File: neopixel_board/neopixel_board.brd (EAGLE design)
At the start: 94 x 86 mm, 64 parts, among them U1 UA7805CKCT, U2 MIC5219, U3 ATMEGA32U4, U4 UA7805CKCT, U5 UA7805CKCT, U6 UA7805CKCT, Y1 16MHz

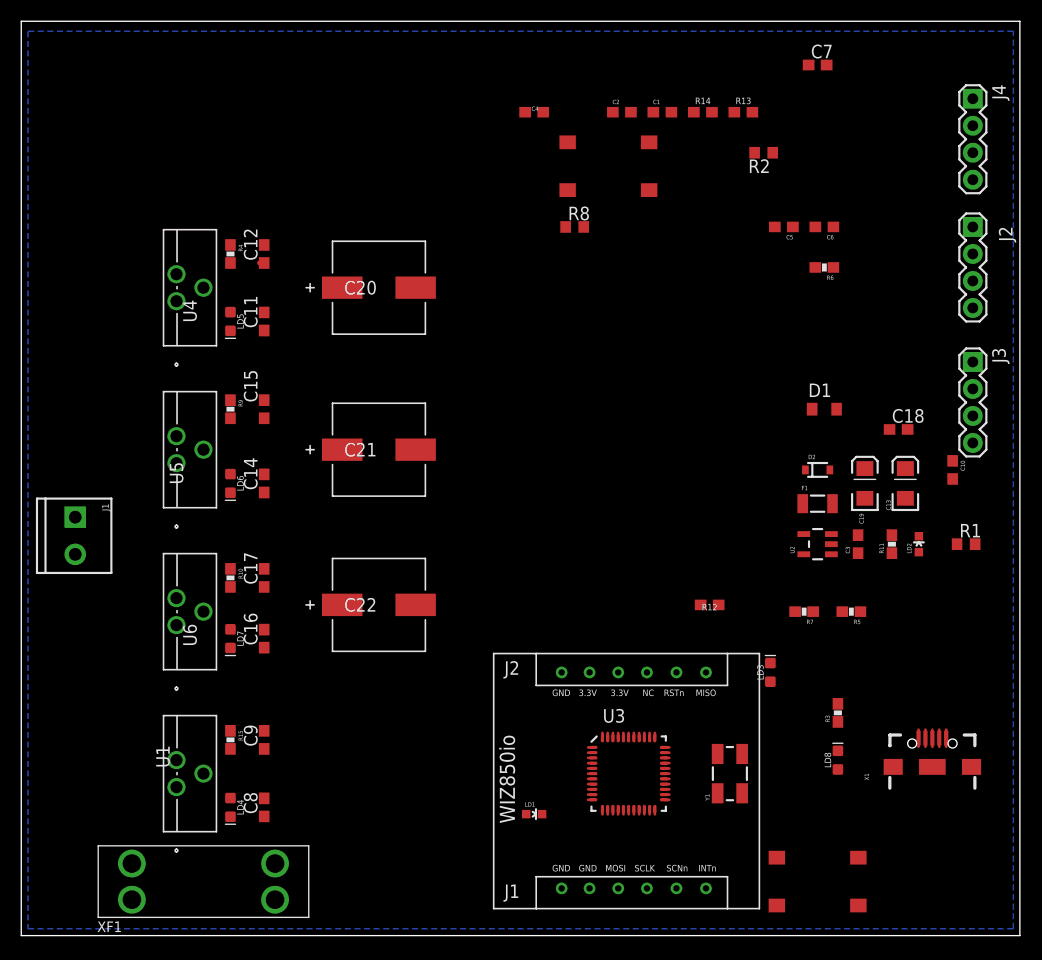
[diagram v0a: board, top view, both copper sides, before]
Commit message: Board Finished (tentative)
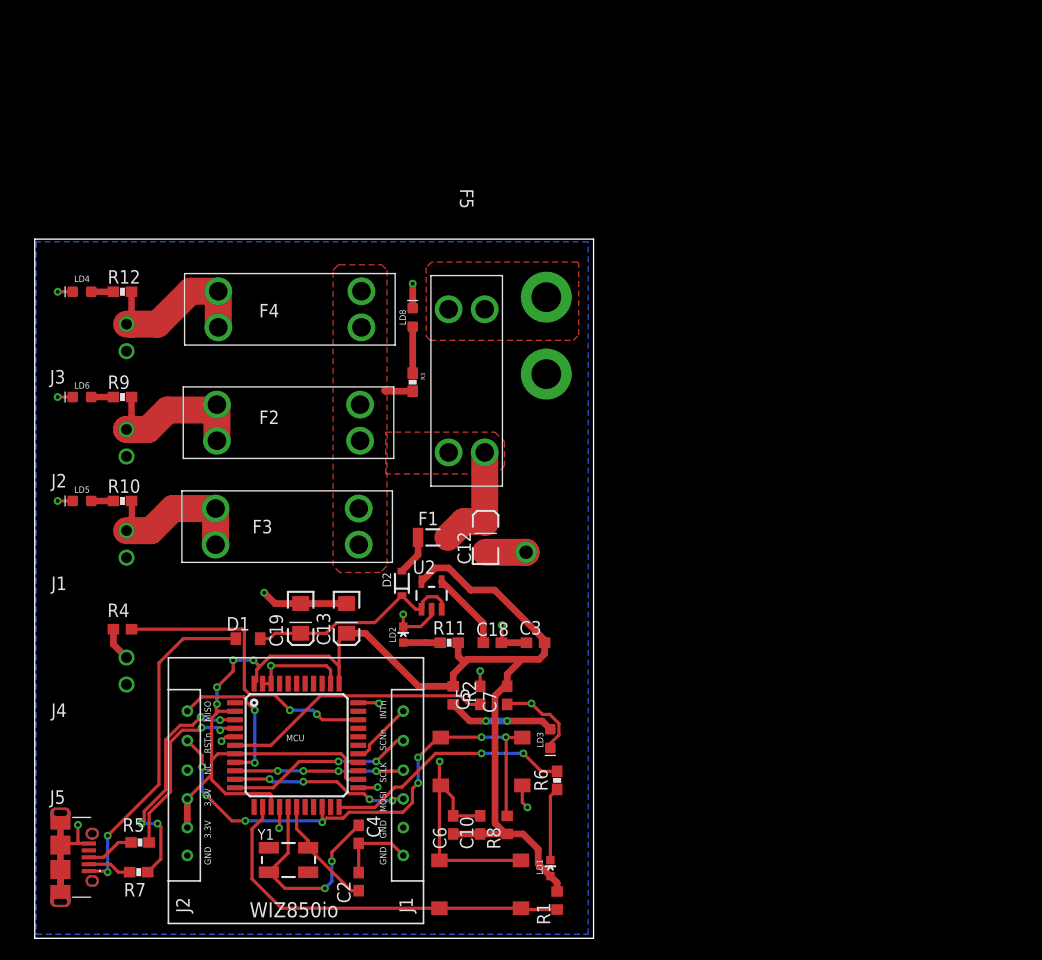
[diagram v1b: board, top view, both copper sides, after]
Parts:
- removed C1: 0.1uF, rcl:C0603
- removed C11, C14, C16, C8: 0.1 uF, rcl:C0603
- removed C15, C17, C9: 0.33 uF, rcl:C0603
- removed C20, C21, C22: 1000uF, neopixel_board:PCAP_8X10-ELECT
- removed LD7: GREEN, SparkFun-LED:LED-0603
- removed R13, R14: 470Ω, SparkFun-Resistors:0603
- removed R15: 1kΩ, SparkFun:0603-RES
- removed U1, U4, U5, U6: UA7805CKCT, Training_Board:KC3
- removed U3: ATMEGA32U4, Testing:QFN-44-NOPAD_1:1-OUTFAKES
- removed X1: (no value), Testing:USB-AB-MICRO-SMD-V03-IN&OUT
- removed XF1: 4A, RoboJackets-Fuses:3557-2
- added 5VSOURCE, GND_TERMINAL: THOLE_SOURCE, neopixel_board:THOLE_SOURCE
- added F2, F3, F4: 4A, neopixel_board:3557-2
- added F5: 13A, neopixel_board:3557-2
- added J5: 47589-0001_2, neopixel_board:MOLEX_47589-0001_FIX
- added MCU: 32U4, SparkFun-IC-Microcontroller:TQFP44
- C12: value 0.33 uF -> 1000uF; device rcl:C0603 -> SparkFun:EIA3216
- J1: value (none) -> SSW-102-02-T-S-RA; device SparkFun-Connectors:SCREWTERMINAL-3.5MM-2 -> neopixel_board:CON2_1X2_TR_SSQ
- J2, J3, J4: value (none) -> SSW-102-02-T-S-RA; device SparkFun-Connectors:1X04 -> neopixel_board:CON2_1X2_TR_SSQ
- R12: value 470Ω -> 1kΩ; device SparkFun-Resistors:0603 -> SparkFun:0603-RES
- R4: value 1kΩ -> 470Ω; device SparkFun:0603-RES -> SparkFun-Resistors:0603
- moved J4 96.1 mm to (9.91, 24.9), turned to 90 degrees
- moved J2 82.2 mm to (9.91, 46.4), turned to 90 degrees
- moved J3 79.7 mm to (9.91, 56.3), turned to 90 degrees
- moved C2 76.5 mm to (31.8, 5.08), turned to 90 degrees
- moved R5 70.4 mm to (11.2, 8.76)
- moved C4 69.9 mm to (31.8, 9.53), turned to 270 degrees
- moved R7 67.2 mm to (11.0, 5.97)
- moved C6 66.2 mm to (40.6, 10.4), turned to 90 degrees
- moved C7 66.1 mm to (45.7, 22.6), turned to 270 degrees
- moved R12 62.6 mm to (9.53, 60.6)
- moved R2 58.8 mm to (40.6, 22.6), turned to 270 degrees
- moved D1 58.4 mm to (21.3, 27.9), turned to 180 degrees
- moved LD8 57.8 mm to (36.8, 58.2)
- moved PB2 57.3 mm to (43.3, 16.4)
- moved R8 56.6 mm to (45.7, 10.4), turned to 90 degrees
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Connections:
- removed net AREF: C1.1, U3.42
- removed net N$3: J4.3, R14.1
- removed net NEOPIXEL_1: R13.2, U3.29
- removed net NEOPIXEL_2: R14.2, U3.30
- removed net UVCC: D1.A, X1.VBUS1
- removed net VCC1: C6.1, C9.1, F1.1, R15.1, U1.3, U3.2, U3.7
- removed net VCC2: C12.1, C20.1, J2.4, R4.1, U4.3
- removed net VCC3: C15.1, C21.1, J3.4, R9.1, U5.3
- removed net VCC4: C17.1, C22.1, J4.4, R10.1, U6.3
- removed net VSOURCE: C11.1, C14.1, C16.1, C8.1, R3.2, U1.1, U4.1, U5.1, U6.1, XF1.3, XF1.4
- new net 5VIN: 5VSOURCE.1, F5.1, F5.2
- new net N$17: D1.A, J5.1
- new net N$18: LD3.A, R2.2
- new net VCC_5V: C12.A, F1.1, F2.3, F2.4, F3.3, F3.4, F4.3, F4.4, F5.3, F5.4, R3.2
- net D+: now also MCU.4; no longer U3.4
- net D-: now also MCU.3; no longer U3.3
- net ETH_INT: now also MCU.27; no longer U3.27
- net ETH_MISO: now also MCU.8; no longer U3.8
- net ETH_MOSI: now also MCU.10; no longer U3.10
- net ETH_RST: now also MCU.20; no longer U3.20
- net ETH_SCK: now also MCU.9; no longer U3.9
- net ETH_SCNN: now also MCU.11; no longer U3.11
- net GND: now also C12.C, GND_TERMINAL.1, J5.5, J5.P$3, J5.P$4, J5.P$5, J5.P$6, MCU.15, MCU.23, MCU.33, MCU.35, MCU.42, MCU.43, MCU.5; no longer C1.2, C11.2, C12.2, C14.2, C15.2, C16.2, C17.2, C20.2, C21.2, C22.2, C8.2, C9.2, J2.2, J3.2, J4.2, LD3.A, LD7.C, R2.2, U1.2, U3.15, U3.23, U3.33, U3.35, U3.43, U3.5, U4.2, U5.2, U6.2, X1.GND1
- net MCU_RST: now also MCU.13; no longer U3.13
- net N$1: now also MCU.16; no longer U3.16
- net N$10: now also F2.1, F2.2, J2.2, R9.2; no longer LD7.A, R10.2
- net N$11: now also F3.1, F3.2, J1.2, R10.2; no longer LD4.A, R15.2
- net N$12: now also F4.1, F4.2, J3.2, R12.2; no longer LD5.A, R4.2
- net N$13: now also J4.2, R4.1; no longer LD6.A, R9.2
- net N$14: now also LD4.A; no longer J2.3
- net N$15: now also LD5.A, R10.1; no longer J3.3, R13.1
- net N$16: now also LD6.A, R9.1; no longer J1.2, XF1.1, XF1.2
- net N$2: now also MCU.17; no longer U3.17
- net N$4: now also MCU.6; no longer U3.6
- net N$6: now also J5.2; no longer X1.D-1
- net N$8: now also J5.3; no longer X1.D+1
- net NEOPIXEL_0: now also MCU.31, R4.2; no longer R12.2, U3.31
- net TXLED: now also MCU.22; no longer U3.22
- net VCC1_3.3V: now also C6.1, MCU.14, MCU.2, MCU.24, MCU.34, MCU.44, MCU.7; no longer U3.14, U3.24, U3.34, U3.44
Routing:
- net VCC1_3.3V: track 0.00 -> 134.1 mm, vias 0 -> 4
- net GND: track 0.00 -> 100.9 mm, vias 0 -> 18
- net ETH_RST: track 0.00 -> 51.0 mm, vias 0 -> 8
- net MCU_RST: track 0.00 -> 37.1 mm
- net N$17: track 0.00 -> 31.7 mm, vias 0 -> 2
- net NEOPIXEL_0: track 0.00 -> 28.1 mm, vias 0 -> 2
- net N$4: track 0.00 -> 25.3 mm
- net TXLED: track 0.00 -> 23.3 mm, vias 0 -> 2
- net D-: track 0.00 -> 23.1 mm, vias 0 -> 4
- net RAW: track 0.00 -> 21.0 mm
- net N$1: track 0.00 -> 20.0 mm, vias 0 -> 2
- net ETH_SCNN: track 0.00 -> 17.7 mm, vias 0 -> 2
- net D+: track 0.00 -> 17.2 mm, vias 0 -> 2
- net ETH_MOSI: track 0.00 -> 16.8 mm, vias 0 -> 4
- net N$10: track 0.00 -> 16.5 mm
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- added copper zone on layer 1, net 5VIN
- added copper zone on layer 1, net VCC_5V
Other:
- board size 94 x 86 mm -> 52.6 x 65.8 mm
